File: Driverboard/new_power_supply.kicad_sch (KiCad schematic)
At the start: 18 parts

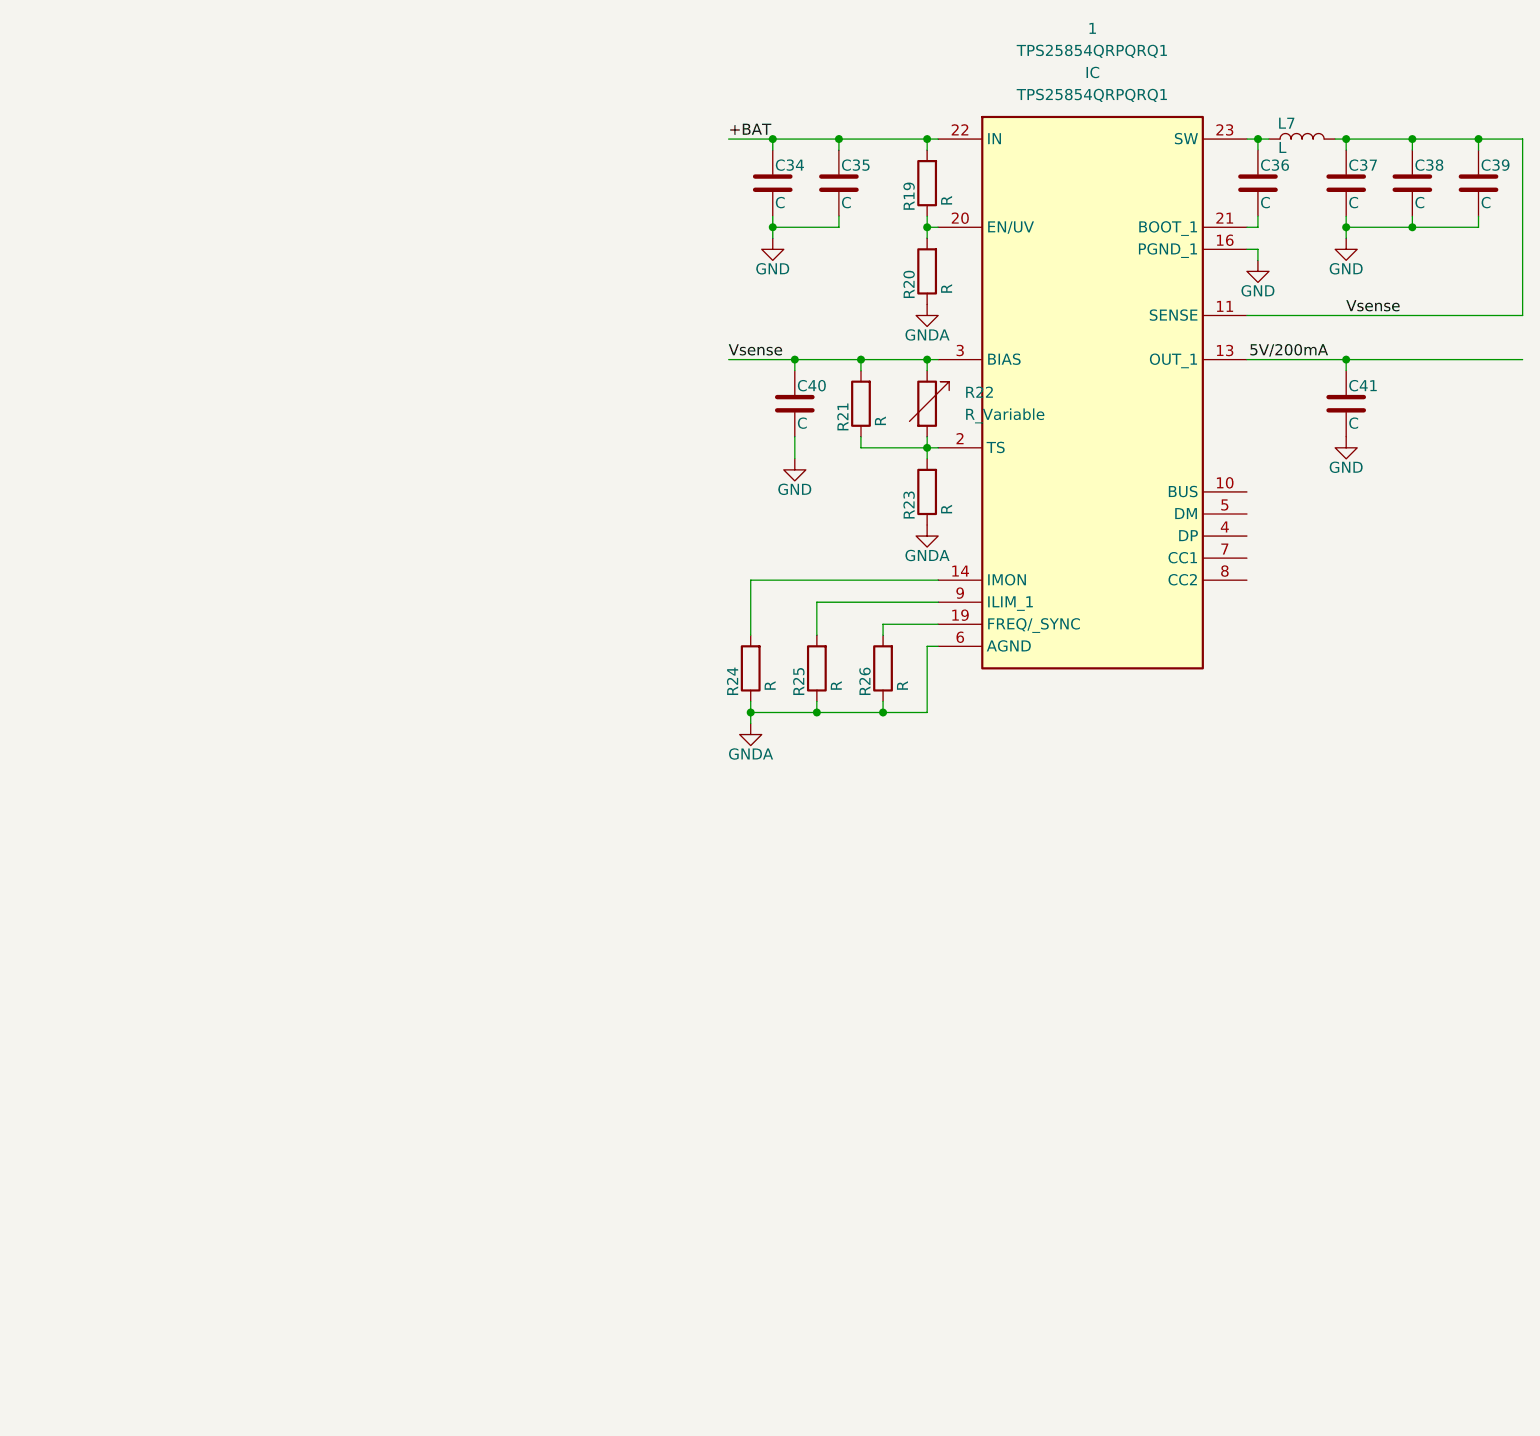
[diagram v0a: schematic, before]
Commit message: WIP
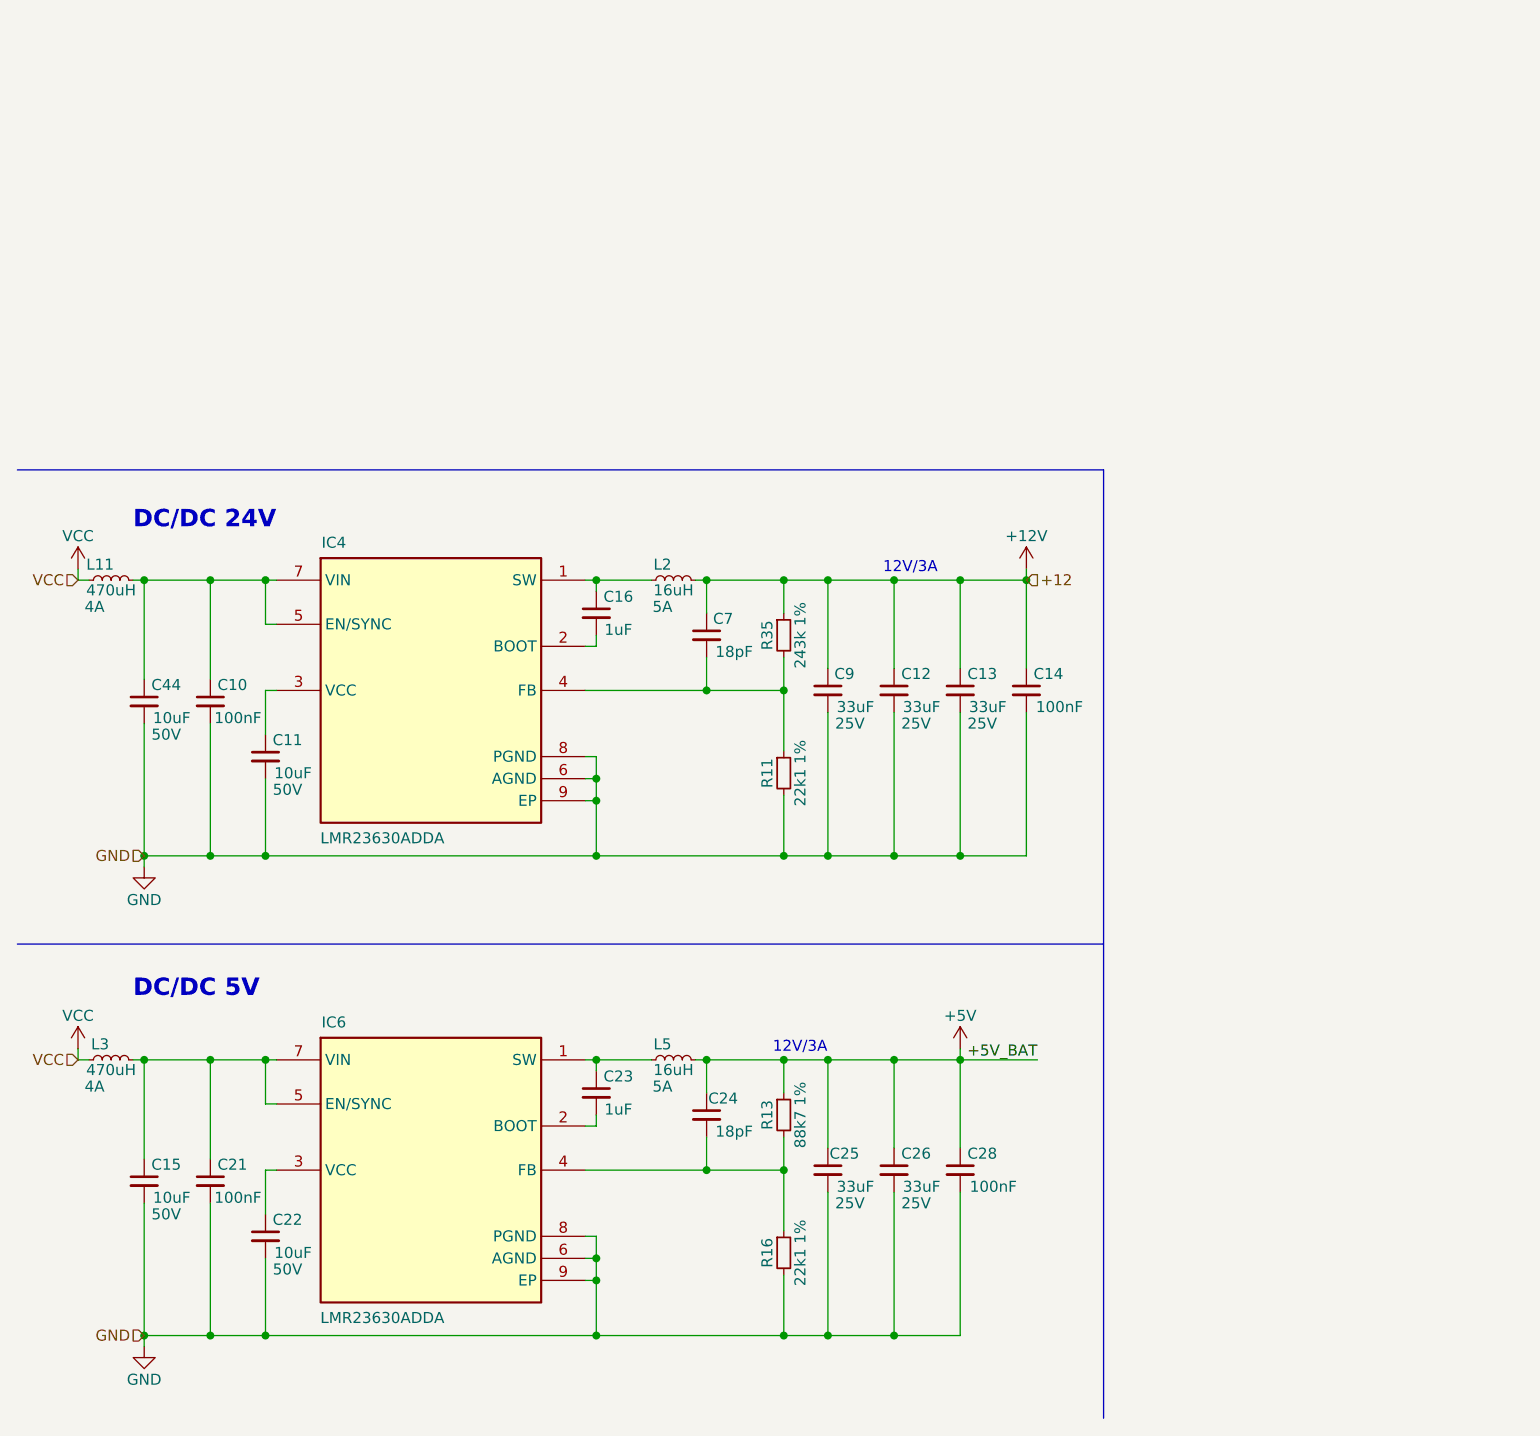
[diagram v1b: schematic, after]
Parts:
- removed 1: TPS25854QRPQRQ1, symbol TPS25854QRPQRQ1:TPS25854QRPQRQ1
- removed C34, C35, C36, C37, C38, C39, C40, C41: C, symbol Device:C
- removed L7: L, symbol Device:L
- removed R19, R20, R21, R23, R24, R25, R26: R, symbol Device:R
- removed R22: R_Variable, symbol Device:R_Variable
- added C10, C14, C21, C28: 100nF, symbol Device:C_Small
- added C11, C15, C22, C44: 10uF, symbol Device:C_Small
- added C12, C13, C25, C26, C9: 33uF, symbol Device:C_Small
- added C16, C23: 1uF, symbol Device:C_Small
- added C24, C7: 18pF, symbol Device:C_Small
- added IC4, IC6: LMR23630ADDA, symbol LMR23630ADDA:LMR23630ADDA
- added L11, L3: 470uH, symbol Device:L_Small
- added L2, L5: 16uH, symbol Device:L_Small
- added R11, R16: 22k1 1%, symbol Device:R_Small
- added R13: 88k7 1%, symbol Device:R_Small
- added R35: 243k 1%, symbol Device:R_Small
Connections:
- net GND: now also C10.2, C11.2, C12.2, C13.2, C14.2, C15.2, C21.2, C22.2, C25.2, C26.2, C28.2, C44.2, C9.2, IC4.6 (AGND), IC4.8 (PGND), IC4.9 (EP), IC6.6 (AGND), IC6.8 (PGND), IC6.9 (EP), R11.2, R16.2
- new net: C7.2, IC4.4 (FB), R11.1, R35.2
- new net: C24.2, IC6.4 (FB), R13.2, R16.1
- new net: C16.1, IC4.1 (SW), L2.1
- new net: C15.1, C21.1, IC6.5 (EN/SYNC), IC6.7 (VIN), L3.2
- new net: C10.1, C44.1, IC4.5 (EN/SYNC), IC4.7 (VIN), L11.2
- new net: C23.1, IC6.1 (SW), L5.1
- new net: C22.1, IC6.3 (VCC)
- new net: C11.1, IC4.3 (VCC)
- new net: C16.2, IC4.2 (BOOT)
- new net: C23.2, IC6.2 (BOOT)
- new net +12V: C12.1, C13.1, C14.1, C7.1, C9.1, L2.2, R35.1
- new net +5V: C24.1, C25.1, C26.1, C28.1, L5.2, R13.1
- new net VCC: L11.1, L3.1
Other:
- note added: "12V/3A"
- note added: "DC/DC 24V"
- note added: "DC/DC 5V"
